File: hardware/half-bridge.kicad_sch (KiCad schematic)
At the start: 30 parts, among them J7 Phase_OUT, Q1 AGM015N10LL, Q2 AGM015N10LL, Q3 AGM015N10LL, Q4 AGM015N10LL, Q5 AGM015N10LL, Q6 AGM015N10LL, U3 IRS21867S, U4 INA240A2D

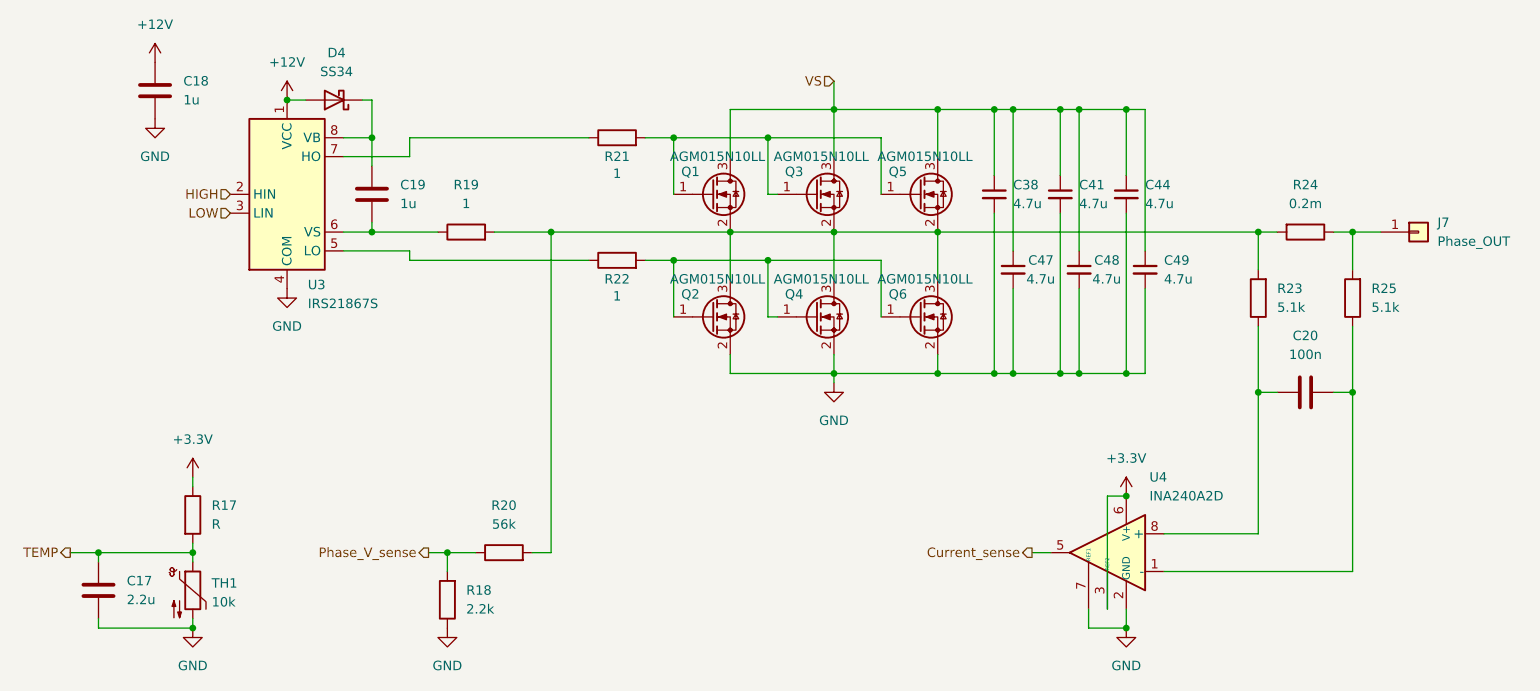
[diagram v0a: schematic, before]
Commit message: Placement study
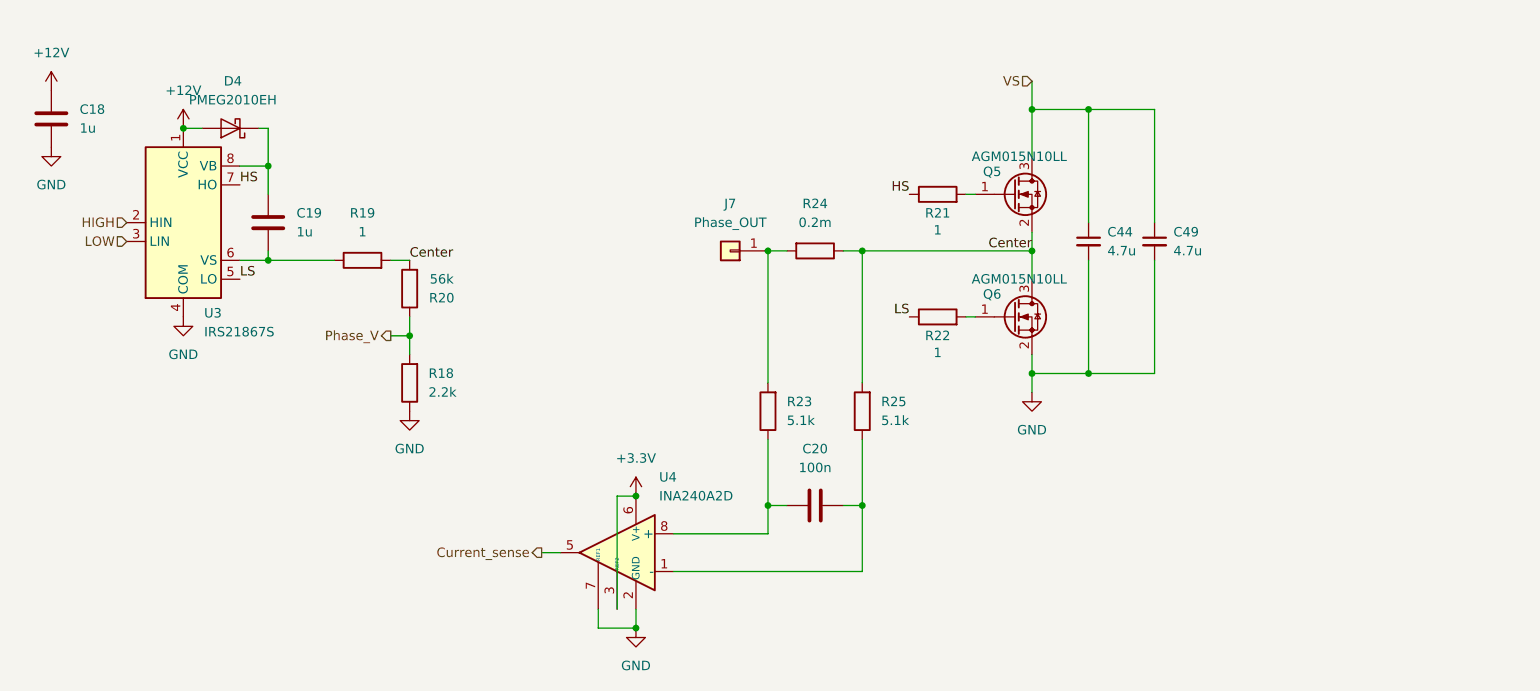
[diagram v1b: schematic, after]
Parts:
- removed C17: 2.2u, symbol Device:C
- removed C38, C41, C47, C48: 4.7u, Capacitor_SMD:C_1210_3225Metric, symbol Device:C_Small
- removed D4: SS34, Diode_SMD:D_SMA, symbol Diode:SS34
- removed Q1, Q2, Q3, Q4: AGM015N10LL, Package_TO_SOT_SMD:Infineon_PG-HSOF-8-1_ThermalVias, symbol Transistor_FET:Q_NMOS_GSD
- removed R17: R, symbol Device:R
- removed TH1: 10k, symbol Device:Thermistor_NTC
- added D4: PMEG2010EH, Diode_SMD:D_SOD-123F, symbol Diode:PMEG2010EH
- C18: footprint (none) -> Capacitor_SMD:C_1206_3216Metric
- C19: footprint (none) -> Capacitor_SMD:C_0805_2012Metric
- C20: footprint (none) -> Capacitor_SMD:C_0402_1005Metric
- C49: footprint Capacitor_SMD:C_1210_3225Metric -> Capacitor_SMD:C_3640_9110Metric
- R18: footprint (none) -> Resistor_SMD:R_0402_1005Metric
- R19, R21, R22: footprint (none) -> Resistor_SMD:R_0805_2012Metric
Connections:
- net +12V: now also D4.2 (A)
- net Center: now reaches Q5.2 (S), Q6.3 (D), R19.2, R20.2
- net Center: now also R24.1, R25.2; no longer R23.2, R24.2
- net LS: now reaches R22.1, U3.5 (LO)
- net HS: now reaches R21.1, U3.7 (HO)
- net at C19.1, U3.8 (VB): now also D4.1 (K)
- net Phase_V_sense renamed Phase_V
- new net: J7.1 (Pin_1), R23.2, R24.2
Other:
- moved on the sheet: C18, C19, C20, C44, C49, J7, Q5, Q6, R18, R19, R20, R21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

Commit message: Power Layout
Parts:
- C49: footprint Capacitor_SMD:C_3640_9110Metric -> Capacitor_SMD:C_1210_3225Metric
- R24: footprint Resistor_SMD:R_4020_10251Metric -> greenmobi:R_3920
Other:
- title: (none) -> GreenMobi Drive
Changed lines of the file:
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@@
 	(generator_version "9.0")
 	(paper "A4")
+	(title_block
+		(title "GreenMobi Drive")
+		(date "2025-07-02")
+		(rev "0.1")
+	)
 	(junction
 		(at 129.54 132.08)
@@
 			)
 		)
-		(property "Footprint" "Resistor_SMD:R_4020_10251Metric"
+		(property "Footprint" "greenmobi:R_3920"
 			(at 153.67 79.502 90)
 			(effects
@@
 			)
 		)
-		(property "Footprint" "Capacitor_SMD:C_3640_9110Metric"
+		(property "Footprint" "Capacitor_SMD:C_1210_3225Metric"
 			(at 199.39 80.01 0)
 			(effects
